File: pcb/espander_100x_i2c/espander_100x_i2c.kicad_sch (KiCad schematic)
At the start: 5 parts, among them J1 DG127A-5.08-06P-14-00AH, J2 DG127A-5.08-06P-14-00AH, J3 DG127A-5.08-06P-14-00AH, J4 DG127A-5.08-06P-14-00AH, U1 MCP23017_SP

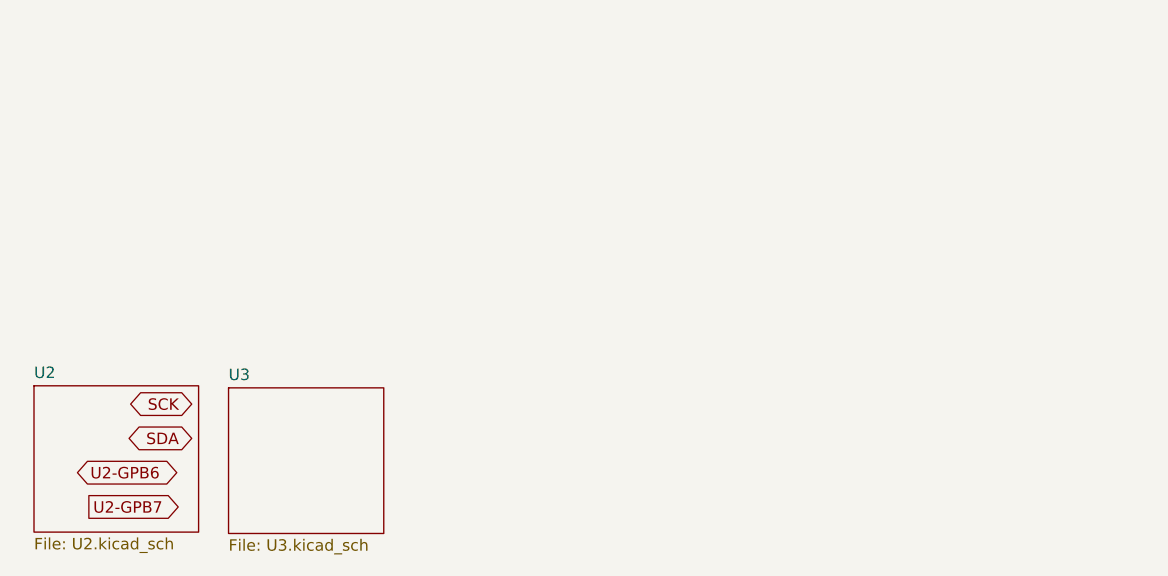
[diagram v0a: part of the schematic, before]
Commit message: Refactor code structure for improved readability and maintainability
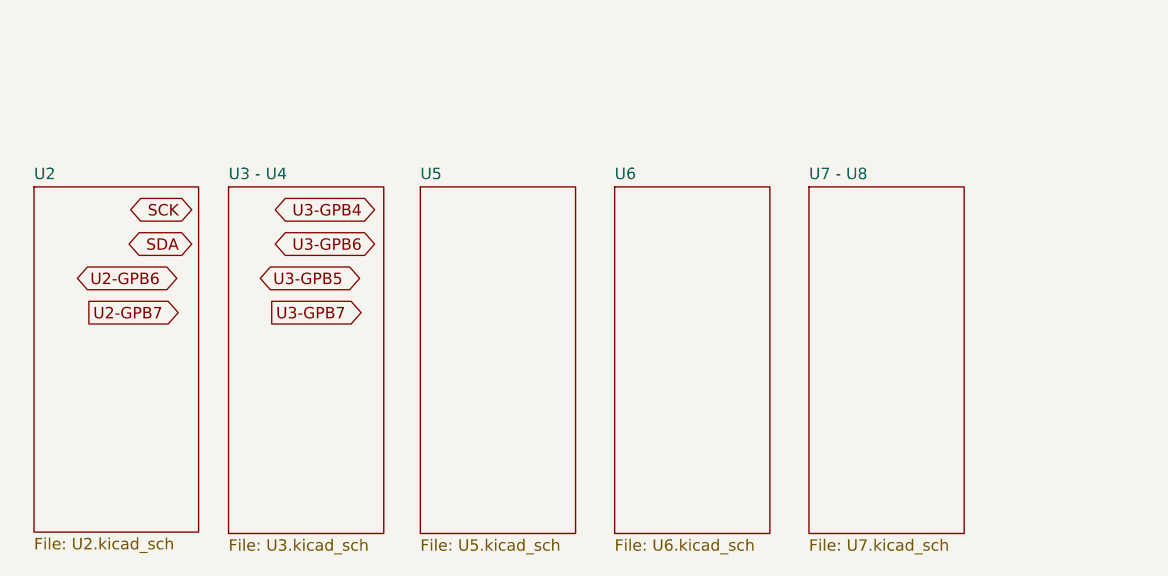
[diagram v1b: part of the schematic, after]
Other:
- sheet U3 renamed U3 - U4
- added sheet U5 (U5.kicad_sch)
- added sheet U6 (U6.kicad_sch)
- added sheet U7 - U8 (U7.kicad_sch)
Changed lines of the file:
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@@
 		)
 	)
-	(global_label "U2-GPB7"
-		(shape output)
-		(at 24.13 191.77 0)
+	(global_label "U3-GPB5"
+		(shape bidirectional)
+		(at 43.18 166.37 0)
 		(fields_autoplaced yes)
 		(effects
@@
 		)
 		(property "Intersheetrefs" "${INTERSHEET_REFS}"
-			(at 36.2471 191.77 0)
+			(at 56.4084 166.37 0)
 			(effects
 				(font
@@
 		)
 	)
-	(global_label "SDA"
+	(global_label "U3-GPB6"
 		(shape bidirectional)
-		(at 35.56 184.15 180)
+		(at 55.88 162.56 180)
 		(fields_autoplaced yes)
 		(effects
@@
 		)
 		(property "Intersheetrefs" "${INTERSHEET_REFS}"
-			(at 27.8954 184.15 0)
+			(at 42.6516 162.56 0)
 			(effects
 				(font
@@
 		)
 	)
-	(global_label "SCK"
-		(shape bidirectional)
-		(at 35.56 180.34 180)
+	(global_label "U2-GPB7"
+		(shape output)
+		(at 24.13 170.18 0)
 		(fields_autoplaced yes)
 		(effects
@@
 				(size 1.27 1.27)
 			)
+			(justify left)
+		)
+		(property "Intersheetrefs" "${INTERSHEET_REFS}"
+			(at 36.2471 170.18 0)
+			(effects
+				(font
+					(size 1.27 1.27)
+				)
+				(justify left)
+				(hide yes)
+			)
+		)
+	)
+	(global_label "U3-GPB7"
+		(shape output)
+		(at 44.45 170.18 0)
+		(fields_autoplaced yes)
+		(effects
+			(font
+				(size 1.27 1.27)
+			)
+			(justify left)
+		)
+		(property "Intersheetrefs" "${INTERSHEET_REFS}"
+			(at 56.5671 170.18 0)
+			(effects
+				(font
+					(size 1.27 1.27)
+				)
+				(justify left)
+				(hide yes)
+			)
+		)
+	)
+	(global_label "SDA"
+		(shape bidirectional)
+		(at 35.56 162.56 180)
+		(fields_autoplaced yes)
+		(effects
+			(font
+				(size 1.27 1.27)
+			)
 			(justify right)
 		)
 		(property "Intersheetrefs" "${INTERSHEET_REFS}"
-			(at 27.714 180.34 0)
+			(at 27.8954 162.56 0)
+			(effects
+				(font
+					(size 1.27 1.27)
+				)
+				(justify right)
+				(hide yes)
+			)
+		)
+	)
+	(global_label "SCK"
+		(shape bidirectional)
+		(at 35.56 158.75 180)
+		(fields_autoplaced yes)
+		(effects
+			(font
+				(size 1.27 1.27)
+			)
+			(justify right)
+		)
+		(property "Intersheetrefs" "${INTERSHEET_REFS}"
+			(at 27.714 158.75 0)
 			(effects
 				(font
@@
 		)
 	)
-	(global_label "U2-GPB6"
+	(global_label "U3-GPB4"
 		(shape bidirectional)
-		(at 22.86 187.96 0)
+		(at 55.88 158.75 180)
 		(fields_autoplaced yes)
 		(effects
@@
 				(size 1.27 1.27)
 			)
+			(justify right)
+		)
+		(property "Intersheetrefs" "${INTERSHEET_REFS}"
+			(at 42.6516 158.75 0)
+			(effects
+				(font
+					(size 1.27 1.27)
+				)
+				(justify right)
+				(hide yes)
+			)
+		)
+	)
+	(global_label "U2-GPB6"
+		(shape bidirectional)
+		(at 22.86 166.37 0)
+		(fields_autoplaced yes)
+		(effects
+			(font
+				(size 1.27 1.27)
+			)
 			(justify left)
 		)
 		(property "Intersheetrefs" "${INTERSHEET_REFS}"
-			(at 36.0884 187.96 0)
+			(at 36.0884 166.37 0)
 			(effects
 				(font
@@
 	)
 	(sheet
-		(at 18.034 178.308)
-		(size 18.288 16.256)
+		(at 18.034 156.21)
+		(size 18.288 38.354)
 		(exclude_from_sim no)
 		(in_bom yes)
@@
 		)
 		(property "Sheetname" "U2"
-			(at 18.034 177.5964 0)
+			(at 18.034 155.4984 0)
 			(effects
 				(font
@@
 	)
 	(sheet
-		(at 39.6494 178.5366)
-		(size 17.2466 16.1798)
+		(at 60.96 156.21)
+		(size 17.2466 38.5064)
 		(exclude_from_sim no)
 		(in_bom yes)
@@
 			(color 0 0 0 0.0000)
 		)
-		(property "Sheetname" "U3"
-			(at 39.6494 177.825 0)
-			(effects
-				(font
+		(property "Sheetname" "U5"
+			(at 60.96 155.4984 0)
+			(effects
+				(font
+					(size 1.27 1.27)
+				)
+				(justify left bottom)
+			)
+		)
+		(property "Sheetfile" "U5.kicad_sch"
+			(at 60.96 195.301 0)
+			(effects
+				(font
+					(size 1.27 1.27)
+				)
+				(justify left top)
+			)
+		)
+		(instances
+			(project "espander_100x_i2c"
+				(path "/824ceec5-564f-405b-8bea-e5a9f7aa2926"
+					(page "4")
+				)
+			)
+		)
+	)
+	(sheet
+		(at 82.55 156.21)
+		(size 17.2466 38.5064)
+		(exclude_from_sim no)
+		(in_bom yes)
+		(on_board yes)
+		(dnp no)
+		(fields_autoplaced yes)
+		(stroke
+			(width 0.1524)
+			(type solid)
+		)
+		(fill
+			(color 0 0 0 0.0000)
+		)
+		(property "Sheetname" "U6"
+			(at 82.55 155.4984 0)
+			(effects
+				(font
+					(size 1.27 1.27)
+				)
+				(justify left bottom)
+			)
+		)
+		(property "Sheetfile" "U6.kicad_sch"
+			(at 82.55 195.301 0)
+			(effects
+				(font
+					(size 1.27 1.27)
+				)
+				(justify left top)
+			)
+		)
+		(instances
+			(project "espander_100x_i2c"
+				(path "/824ceec5-564f-405b-8bea-e5a9f7aa2926"
+					(page "5")
+				)
+			)
+		)
+	)
+	(sheet
+		(at 104.14 156.21)
+		(size 17.2466 38.5064)
+		(exclude_from_sim no)
+		(in_bom yes)
+		(on_board yes)
+		(dnp no)
+		(fields_autoplaced yes)
+		(stroke
+			(width 0.1524)
+			(type solid)
+		)
+		(fill
+			(color 0 0 0 0.0000)
+		)
+		(property "Sheetname" "U7 - U8"
+			(at 104.14 155.4984 0)
+			(effects
+				(font
+					(size 1.27 1.27)
+				)
+				(justify left bottom)
+			)
+		)
+		(property "Sheetfile" "U7.kicad_sch"
+			(at 104.14 195.301 0)
+			(effects
+				(font
+					(size 1.27 1.27)
+				)
+				(justify left top)
+			)
+		)
+		(instances
+			(project "espander_100x_i2c"
+				(path "/824ceec5-564f-405b-8bea-e5a9f7aa2926"
+					(page "6")
+				)
+			)
+		)
+	)
+	(sheet
+		(at 39.6494 156.21)
+		(size 17.2466 38.5064)
+		(exclude_from_sim no)
+		(in_bom yes)
+		(on_board yes)
+		(dnp no)
+		(fields_autoplaced yes)
+		(stroke
+			(width 0.1524)
+			(type solid)
+		)
+		(fill
+			(color 0 0 0 0.0000)
+		)
+		(property "Sheetname" "U3 - U4"
+			(at 39.6494 155.4984 0)
+			(effects
+				(font
